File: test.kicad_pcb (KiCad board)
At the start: 2 copper layers, 39 parts, among them IC1 BQ24074RGTR, IC2 USBLC6-2SC6, IC3 ESP32-S3-WROOM-1-N16, J1 UART0, J2 73100-0105, J3 73100-0105, SW1 Reset, SW2 Boot, U1 USB-TYPE-C-018, U2 1043, U3 LD1086DT33TR, U4 LD1086DT33TR

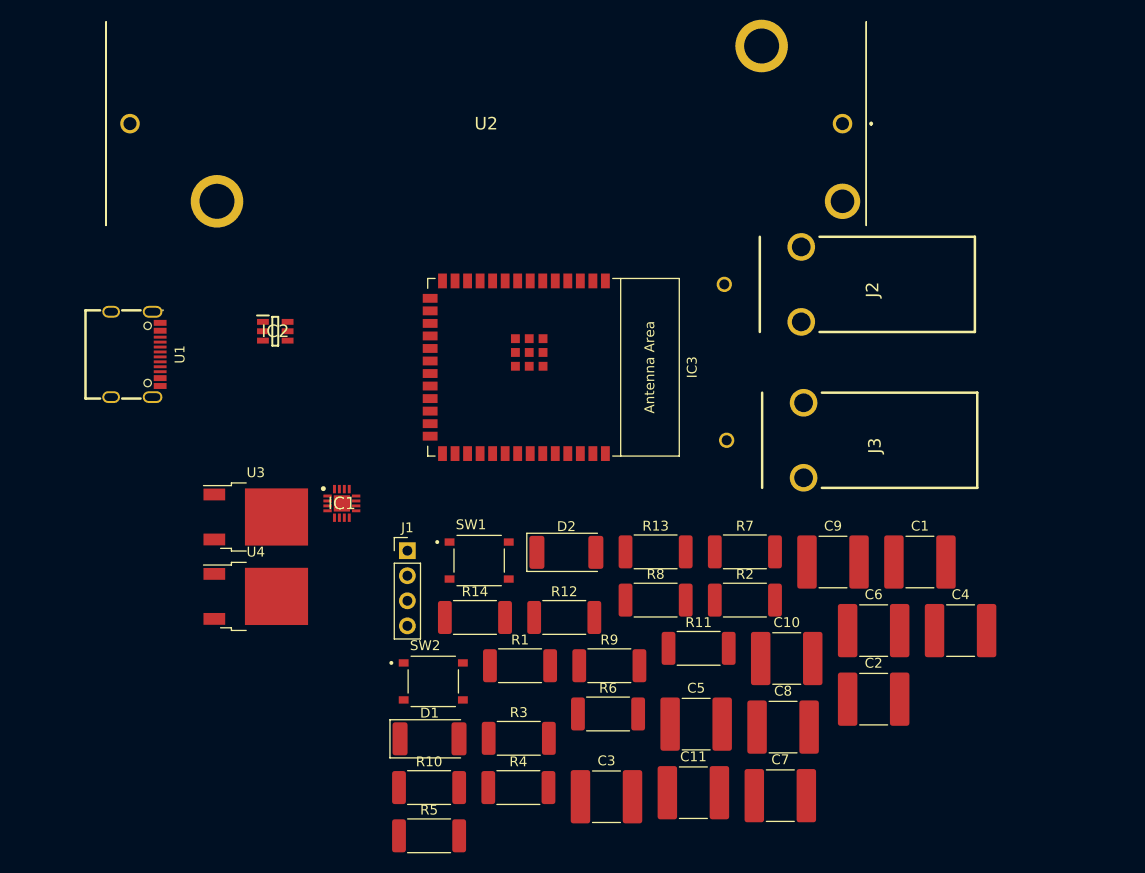
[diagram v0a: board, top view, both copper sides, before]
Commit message: first try of front end
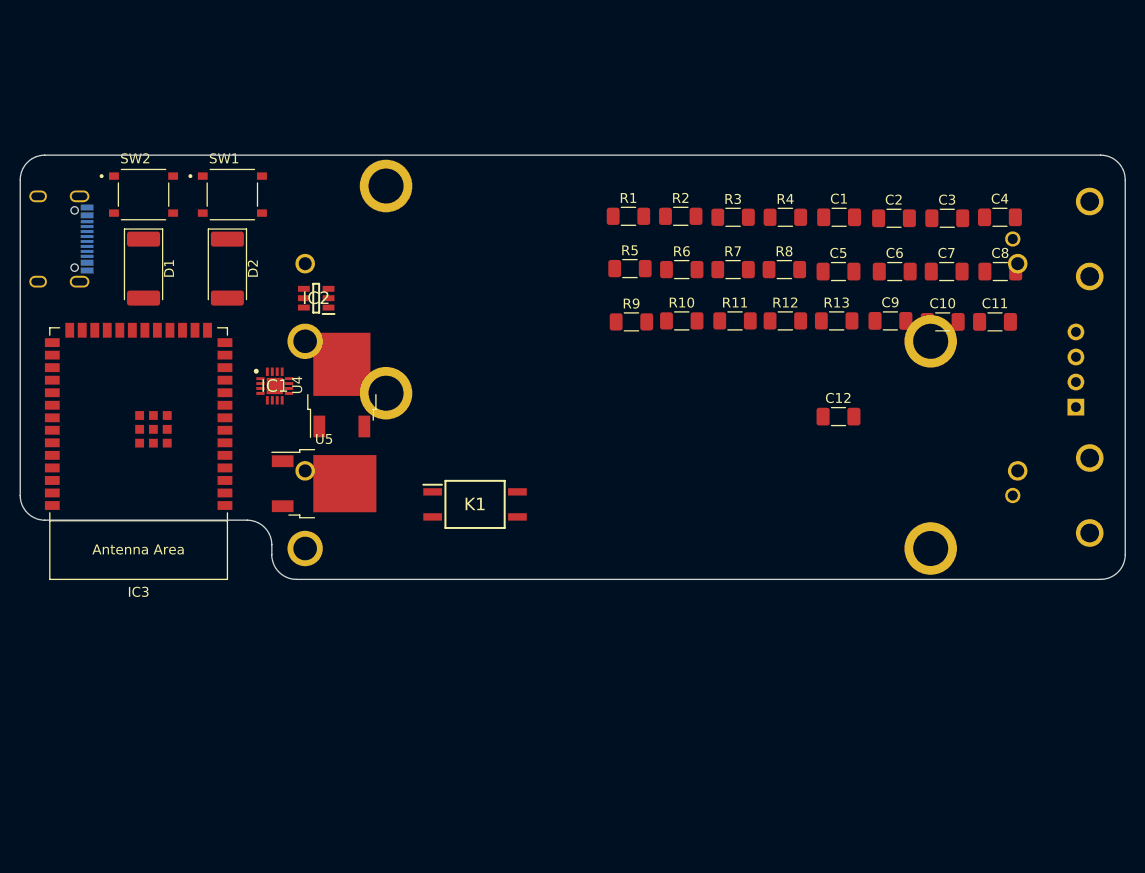
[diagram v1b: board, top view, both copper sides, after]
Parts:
- removed the R3 at (78.5, 149.1)
- added C12: 10u, Capacitor_SMD:C_1206_3216Metric_Pad1.33x1.80mm_HandSolder, F.Cu at (110.9, 116.5)
- added K1: AQY210EHA, project_library:AQY210EHAX, F.Cu at (74.1, 125.4)
- added U2: 1043, project_library:1043, B.Cu at (56.9, 101.0)
- C1, C10, C11, C2, C3, C4, C5, C6, C7, C8, C9: footprint Capacitor_SMD:C_2220_5650Metric_Pad1.97x5.40mm_HandSolder -> Capacitor_SMD:C_1206_3216Metric_Pad1.33x1.80mm_HandSolder
- D1: value LED_PowerOn -> LED_PowerOn?
- IC1: value BQ24074RGTR -> QFN50P300X300X100-17N-D
- IC2: value USBLC6-2SC6 -> SOT95P280X145-6N
- J1, J2, J3: moved to B.Cu
- R1, R2, R4, R7: footprint Resistor_SMD:R_2512_6332Metric_Pad1.40x3.35mm_HandSolder -> Resistor_SMD:R_1206_3216Metric_Pad1.30x1.75mm_HandSolder
- R10: renamed from R11; footprint Resistor_SMD:R_2512_6332Metric_Pad1.40x3.35mm_HandSolder -> Resistor_SMD:R_1206_3216Metric_Pad1.30x1.75mm_HandSolder
- R11: renamed from R12; footprint Resistor_SMD:R_2512_6332Metric_Pad1.40x3.35mm_HandSolder -> Resistor_SMD:R_1206_3216Metric_Pad1.30x1.75mm_HandSolder
- R12: renamed from R13; footprint Resistor_SMD:R_2512_6332Metric_Pad1.40x3.35mm_HandSolder -> Resistor_SMD:R_1206_3216Metric_Pad1.30x1.75mm_HandSolder
- R13: renamed from R14; footprint Resistor_SMD:R_2512_6332Metric_Pad1.40x3.35mm_HandSolder -> Resistor_SMD:R_1206_3216Metric_Pad1.30x1.75mm_HandSolder
- R3: renamed from R6; value 4k12 -> 1k; footprint Resistor_SMD:R_2512_6332Metric_Pad1.40x3.35mm_HandSolder -> Resistor_SMD:R_1206_3216Metric_Pad1.30x1.75mm_HandSolder
- R5: renamed from R8; value 4k12 -> 820; footprint Resistor_SMD:R_2512_6332Metric_Pad1.40x3.35mm_HandSolder -> Resistor_SMD:R_1206_3216Metric_Pad1.30x1.75mm_HandSolder
- R6: renamed from R5; footprint Resistor_SMD:R_2512_6332Metric_Pad1.40x3.35mm_HandSolder -> Resistor_SMD:R_1206_3216Metric_Pad1.30x1.75mm_HandSolder
- R8: renamed from R9; footprint Resistor_SMD:R_2512_6332Metric_Pad1.40x3.35mm_HandSolder -> Resistor_SMD:R_1206_3216Metric_Pad1.30x1.75mm_HandSolder
- R9: renamed from R10; footprint Resistor_SMD:R_2512_6332Metric_Pad1.40x3.35mm_HandSolder -> Resistor_SMD:R_1206_3216Metric_Pad1.30x1.75mm_HandSolder
- U1: value USB-TYPE-C-018 -> USB-C_SMD-TYPE-C-31-M-12; moved to B.Cu
- U3: renamed from U2; moved to B.Cu
- moved J1 69.3 mm to (135.0, 115.5)
- moved C3 68.0 mm to (122.0, 96.4)
- moved U3 64.8 mm to (56.9, 122.0), turned to 180 degrees
- moved R4 63.8 mm to (105.5, 96.3)
- moved R6 62.8 mm to (95.0, 101.6)
- moved SW2 57.4 mm to (40.5, 94.0)
- moved C11 56.7 mm to (126.8, 106.9)
- moved D1 55.8 mm to (40.5, 101.5), turned to -90 degrees
- moved C7 55.7 mm to (121.9, 101.8)
- moved R3 51.9 mm to (100.2, 96.3)
- moved R9 51.5 mm to (90.0, 106.9)
- moved C8 51.2 mm to (127.3, 101.8)
- moved C2 48.8 mm to (116.6, 96.4)
- moved C5 48.1 mm to (110.9, 101.8)
- moved R13 47.4 mm to (110.8, 106.8)
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- renumbered U3 to U4, U4 to U5
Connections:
- IC1 pad 15: Net-(IC1-Pad15) -> GND
- IC2 pad 4: /USB_D+ -> Net-(IC2-Pad4)
- IC2 pad 6: /USB_D- -> Net-(IC2-Pad6)
- IC3 pad 20: unconnected-(IC3-Pad20) -> /MISO
- IC3 pad 21: unconnected-(IC3-Pad21) -> /MOSI
- IC3 pad 22: unconnected-(IC3-Pad22) -> /SCLK
- IC3 pad 8: unconnected-(IC3-Pad8) -> /CS
- U1 pad A6: /USB_D+ -> Net-(IC2-Pad4)
- U1 pad A7: /USB_D- -> Net-(IC2-Pad6)
- U1 pad B6: /USB_D+ -> Net-(IC2-Pad4)
- U1 pad B7: /USB_D- -> Net-(IC2-Pad6)
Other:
- board outline added: 112 x 43 mm
